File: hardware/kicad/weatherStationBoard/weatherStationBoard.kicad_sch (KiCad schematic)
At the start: 3 parts, among them P1 USB_C_Plug_USB2.0

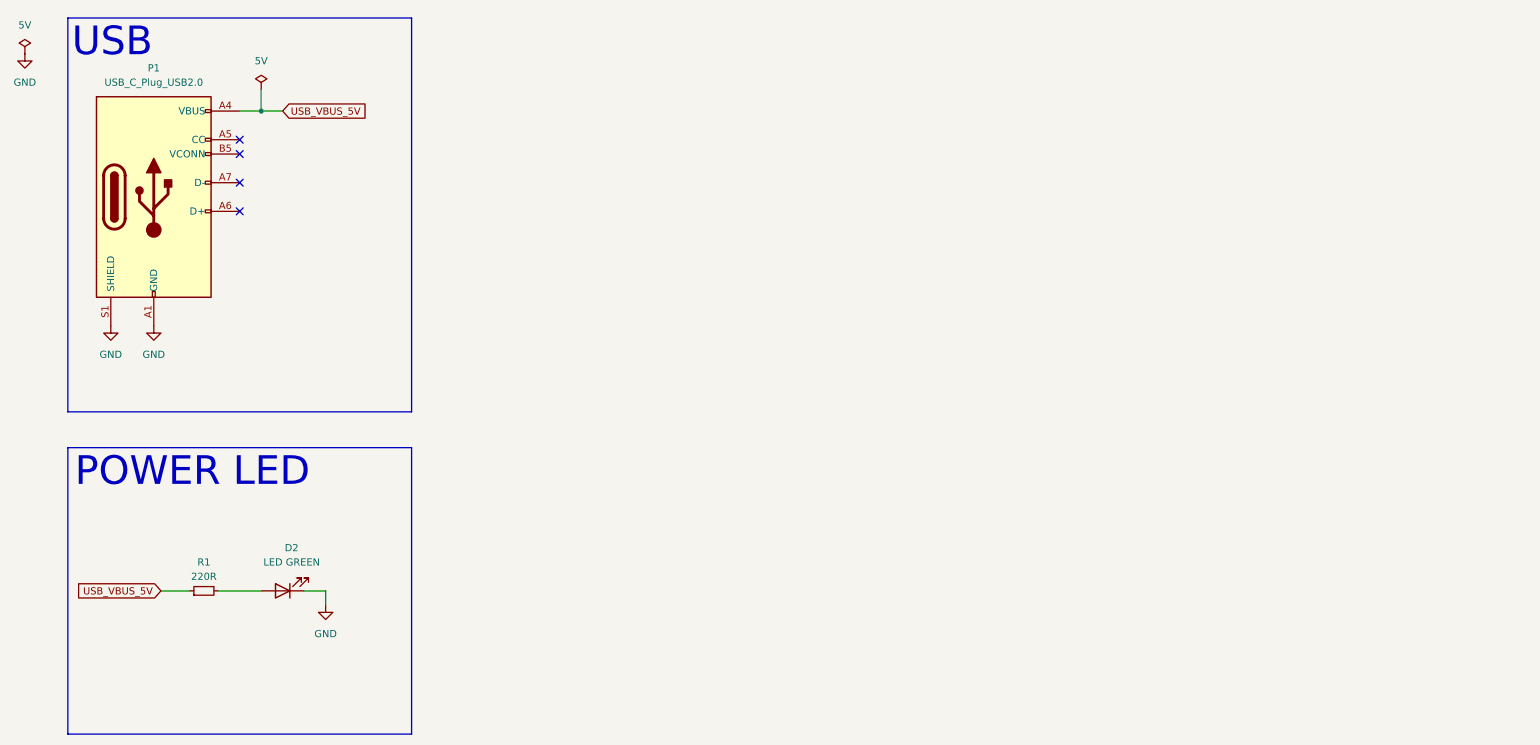
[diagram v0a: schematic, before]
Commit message: power, 5vto3v, usb to serial
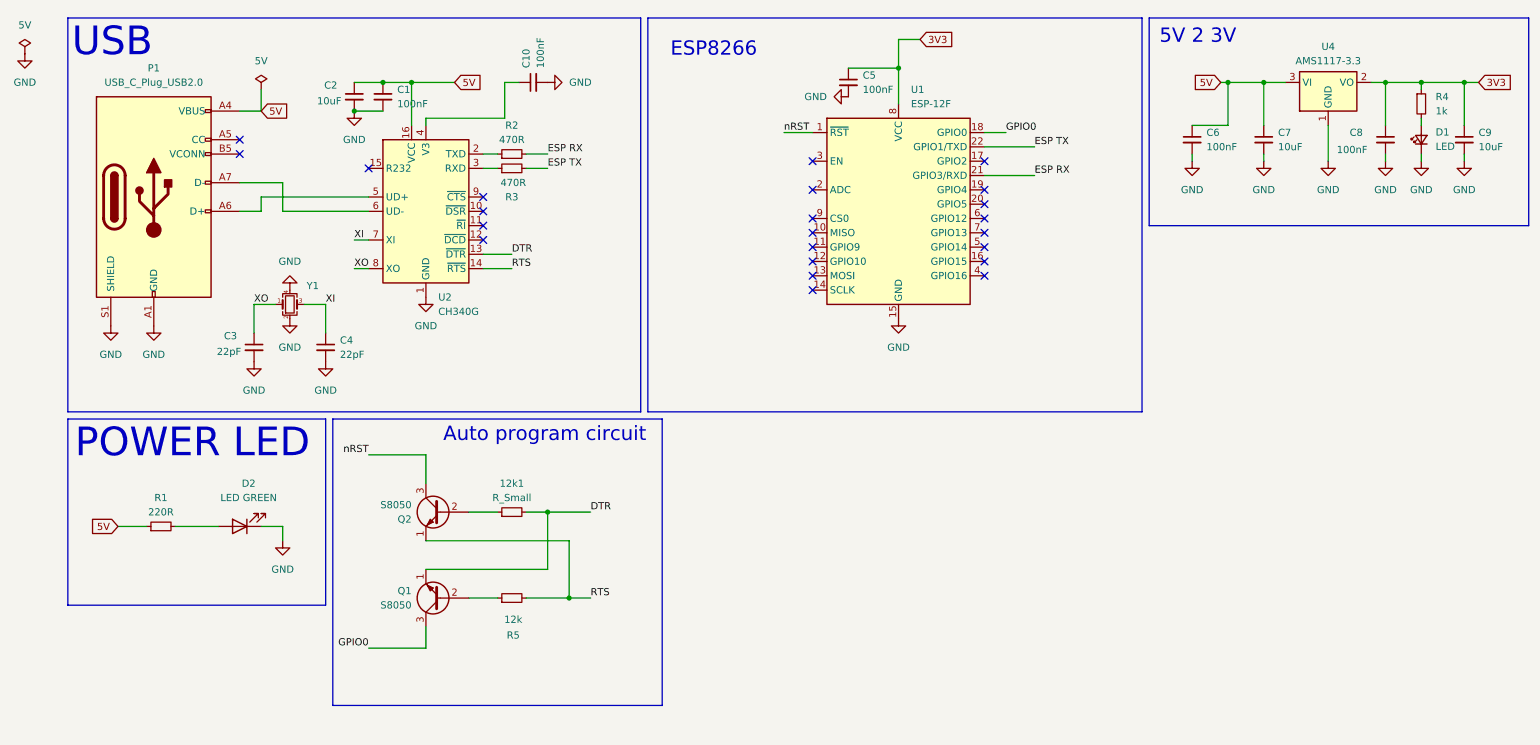
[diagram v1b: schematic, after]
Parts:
- added 12k1: R_Small, Resistor_SMD:R_0805_2012Metric, symbol Device:R_Small
- added C1, C10, C5, C6, C8: 100nF, Capacitor_SMD:C_0805_2012Metric, symbol Device:C_Small
- added C2, C7, C9: 10uF, Capacitor_SMD:C_0805_2012Metric, symbol Device:C_Small
- added C3, C4: 22pF, Capacitor_SMD:C_0805_2012Metric, symbol Device:C_Small
- added D1: LED, LED_SMD:LED_0805_2012Metric, symbol Device:LED_Small
- added Q1, Q2: S8050, Package_TO_SOT_THT:TO-92_Inline, symbol Transistor_BJT:S8050
- added R2, R3: 470R, Resistor_SMD:R_0805_2012Metric, symbol Device:R_Small
- added R4: 1k, Resistor_SMD:R_0805_2012Metric, symbol Device:R_Small
- added R5: 12k, Resistor_SMD:R_0805_2012Metric, symbol Device:R_Small
- added U1: ESP-12F, RF_Module:ESP-12E, symbol RF_Module:ESP-12F
- added U2: CH340G, Package_SO:SOIC-16_3.9x9.9mm_P1.27mm, symbol Interface_USB:CH340G
- added U4: AMS1117-3.3, Package_TO_SOT_SMD:SOT-223-3_TabPin2, symbol Regulator_Linear:AMS1117-3.3
- added Y1: Crystal_GND24_Small, Crystal:Crystal_SMD_3225-4Pin_3.2x2.5mm, symbol Device:Crystal_GND24_Small
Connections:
- net GND: now also C1.2, C10.2, C2.2, C3.2, C4.2, C5.2, C6.2, C7.2, C8.2, C9.2, D1.1 (K), U1.15 (GND), U2.1 (GND), U4.1 (GND), Y1.2, Y1.4
- net at P1.A6 (D+): now also U2.5 (UD+)
- net at P1.A7 (D-): now also U2.6 (UD-)
- net USB_VBUS_5V renamed 5V
- net 5V: now also C1.1, C2.1, C6.1, C7.1, U2.16 (VCC), U4.3 (VI)
- new net: R3.1, U2.3 (RXD)
- new net: D1.2 (A), R4.2
- new net: 12k1.1, Q2.2 (B)
- new net: R2.1, U2.2 (TXD)
- new net: Q1.2 (B), R5.1
- new net: C10.1, U2.4 (V3)
- new net 3V3: C5.1, C8.1, C9.1, R4.1, U1.8 (VCC), U4.2 (VO)
- new net DTR: 12k1.2, Q1.1 (E), U2.13 (~{DTR})
- new net ESP RX: R2.2, U1.21 (GPIO3/RXD)
- new net ESP TX: R3.2, U1.22 (GPIO1/TXD)
- new net GPIO0: Q1.3 (C), U1.18 (GPIO0)
- new net RTS: Q2.1 (E), R5.2, U2.14 (~{RTS})
- new net XI: C4.1, U2.7 (XI), Y1.3
- new net XO: C3.1, U2.8 (XO), Y1.1
- new net nRST: Q2.3 (C), U1.1 (~{RST})
- no-connect marks 4 -> 23
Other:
- note added: "5V 2 3V"
- note added: "Auto program circuit"
- note added: "ESP8266"
- moved on the sheet: D2, R1
